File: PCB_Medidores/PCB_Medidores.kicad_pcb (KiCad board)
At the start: 2 copper layers, 85 x 56 mm, 20 parts, among them SW1 SW_Push, U1 SENO, U2 tp4056, U3 DS18B20, U4 ATmega8L-8PU, U5 EL814, U6 NRF24L01_Breakout, Y1 16MHz

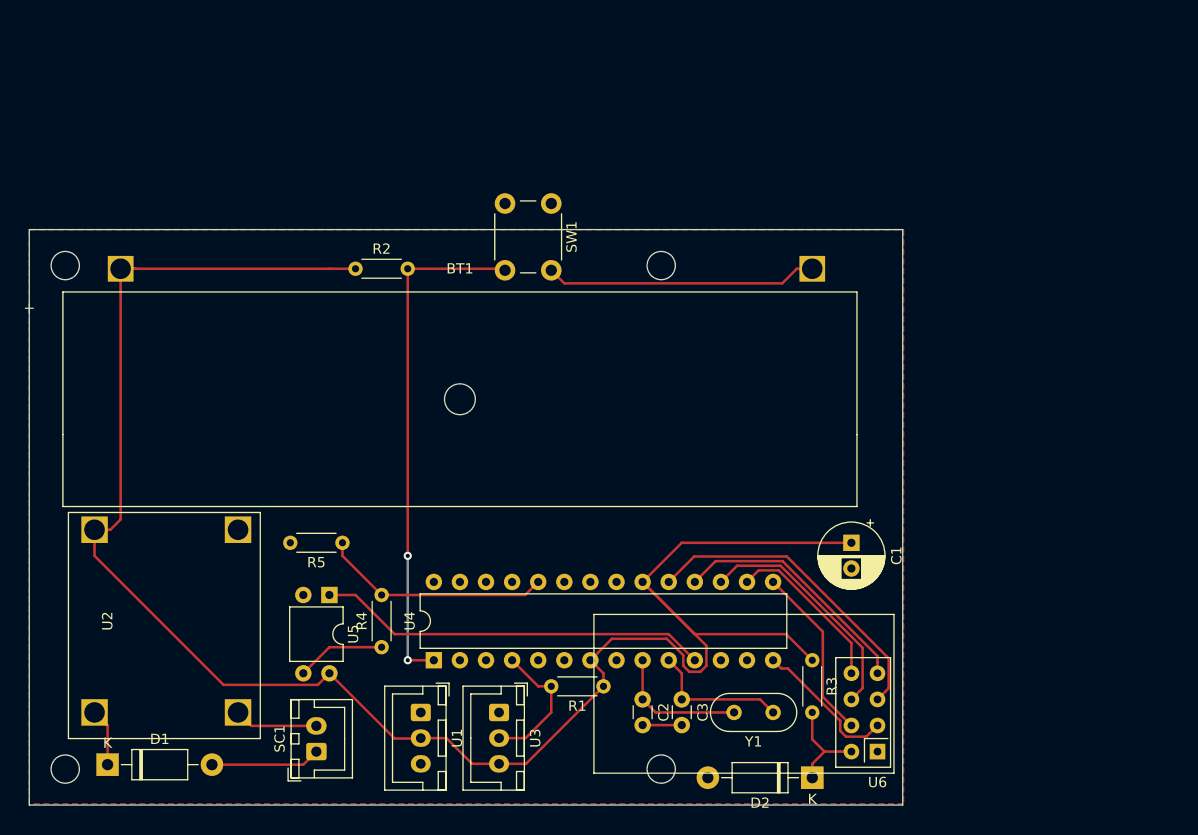
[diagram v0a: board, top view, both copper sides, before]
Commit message: [PCB Medidores e Correção]
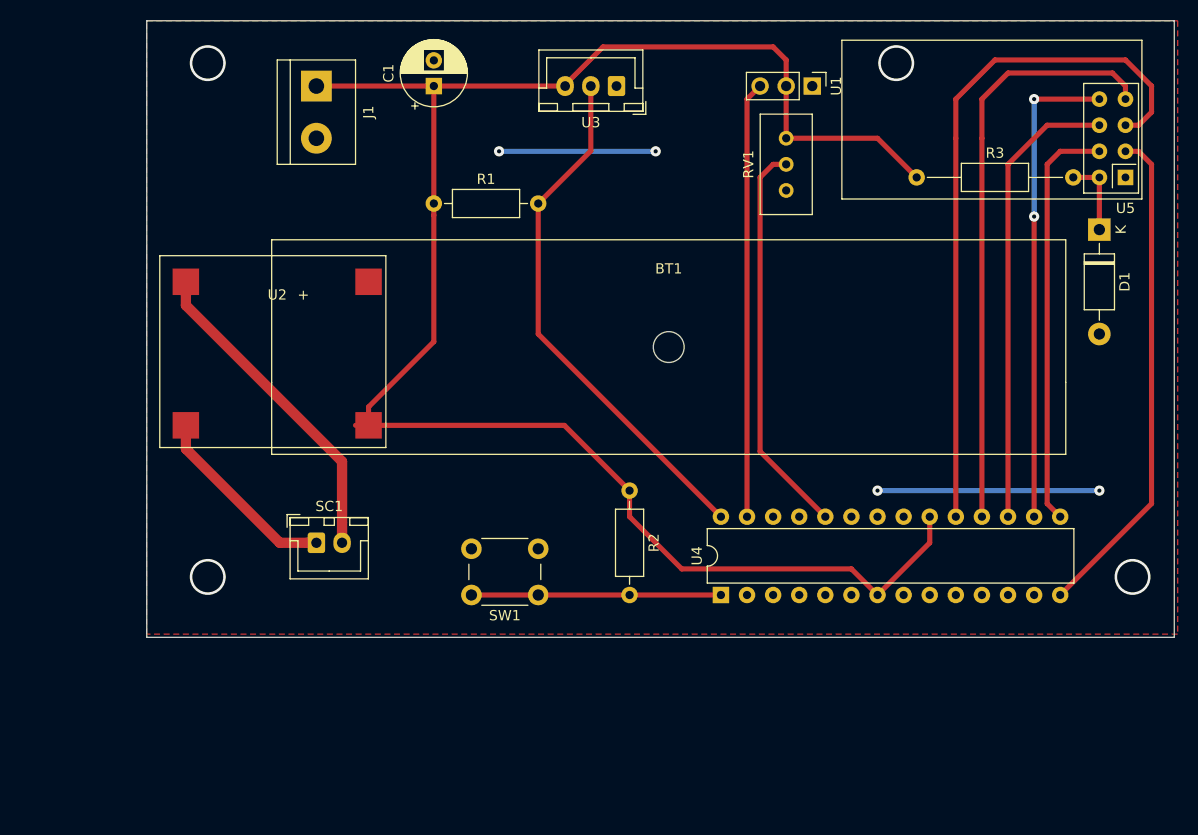
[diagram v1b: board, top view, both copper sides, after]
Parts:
- removed C2, C3: 22pF, Capacitor_THT:C_Disc_D3.0mm_W1.6mm_P2.50mm
- removed D2: 1N4728, Diode_THT:D_DO-41_SOD81_P10.16mm_Horizontal
- removed R4: 10k, Resistor_THT:R_Axial_DIN0204_L3.6mm_D1.6mm_P5.08mm_Horizontal
- removed R5: 33k, Resistor_THT:R_Axial_DIN0204_L3.6mm_D1.6mm_P5.08mm_Horizontal
- removed U6: NRF24L01_Breakout, RF_Module:nRF24L01_Breakout
- removed Y1: 16MHz, Crystal:Crystal_HC52-6mm_Vertical
- added J1: Screw_Terminal_01x02, TerminalBlock:TerminalBlock_bornier-2_P5.08mm, F.Cu at (115.6, 62.2)
- added RV1: R_POT_TRIM, Potentiometer_THT:Potentiometer_Bourns_3296W_Vertical, F.Cu at (161.3, 67.3)
- D1: value 1N4007 -> 1N4728
- R1, R2: footprint Resistor_THT:R_Axial_DIN0204_L3.6mm_D1.6mm_P5.08mm_Horizontal -> Resistor_THT:R_Axial_DIN0207_L6.3mm_D2.5mm_P10.16mm_Horizontal
- R3: footprint Resistor_THT:R_Axial_DIN0204_L3.6mm_D1.6mm_P5.08mm_Horizontal -> Resistor_THT:R_Axial_DIN0207_L6.3mm_D2.5mm_P15.24mm_Horizontal
- SW1: footprint Button_Switch_THT:SW_PUSH_6mm_H5mm -> Button_Switch_THT:SW_PUSH_6mm_H4.3mm
- U1: footprint Connector_JST:JST_XH_B3B-XH-A_1x03_P2.50mm_Vertical -> Connector_PinHeader_2.54mm:PinHeader_1x03_P2.54mm_Vertical
- U4: value ATmega8L-8PU -> ATmega328P-PU
- U5: value EL814 -> NRF24L01_Breakout; footprint Package_DIP:DIP-4_W7.62mm -> RF_Module:nRF24L01_Breakout
- moved D1 109.7 mm to (191.8, 76.2), turned to 270 degrees
- moved U5 87.5 mm to (194.3, 71.1), turned to 180 degrees
- moved U1 71.9 mm to (163.8, 62.2)
- moved U3 62.0 mm to (144.8, 62.2), turned to 180 degrees
- moved C1 60.2 mm to (127.0, 62.2), turned to 90 degrees
- moved R1 49.8 mm to (127.0, 73.7), turned to 0 degrees
- moved R3 48.1 mm to (174.0, 71.1), turned to 0 degrees
- moved U2 41.5 mm to (110.5, 78.7), turned to 0 degrees
- moved SW1 38.1 mm to (137.2, 111.8), turned to 180 degrees
- moved R2 34.3 mm to (146.1, 101.6), turned to 270 degrees
- moved U4 28.7 mm to (154.9, 111.8)
- moved BT1 20.9 mm to (149.9, 82.5)
- moved SC1 20.3 mm to (115.6, 106.7), turned to 0 degrees
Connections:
- D1 pad 2: Net-(D1-Pad2) -> GND
- R3 pad 2: Net-(D2-Pad1) -> Net-(D1-Pad1)
- SC1 pad 1: Net-(D1-Pad2) -> Net-(SC1-Pad1)
- SW1 pad 1: GND -> Net-(R2-Pad2)
- SW1 pad 2: Net-(R2-Pad2) -> GND
- U1 pad 3: Net-(U1-Pad3) -> A0
- U2 pad 1: Net-(D1-Pad1) -> Net-(SC1-Pad1)
- U4 pad 11: AT05 -> Net-(U4-Pad11)
- U4 pad 12: AT06 -> Net-(U4-Pad12)
- U4 pad 23: A0 -> Net-(U4-Pad23)
- U4 pad 27: Net-(U4-Pad27) -> A0
- U4 pad 28: Net-(U4-Pad28) -> AT02
- U4 pad 4: AT02 -> AT05
- U4 pad 5: Net-(U4-Pad5) -> AT06
- U5 pad 1: AT05 -> GND
- U5 pad 2: GND -> Net-(D1-Pad1)
- U5 pad 3: Net-(R4-Pad1) -> AT08
- U5 pad 4: +3V8 -> AT09
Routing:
- net A0: track 0.00 -> 42.4 mm
- net AT05: track 38.2 -> 0.00 mm
- net AT02: track 13.7 -> 51.4 mm
- net AT13: track 31.0 -> 67.9 mm
- net AT08: track 14.3 -> 48.7 mm
- net AT12: track 24.1 -> 57.5 mm
- net AT10: track 16.5 -> 47.0 mm, vias 0 -> 2
- net Net-(R2-Pad2): track 50.2 -> 24.3 mm, vias 2 -> 0
- net Net-(SC1-Pad2): track 8.16 -> 31.9 mm
- net AT09: track 17.1 -> 40.4 mm
- net AT11: track 23.2 -> 44.8 mm
- net Net-(SC1-Pad1): track 0.00 -> 18.8 mm
- net A1: track 22.4 -> 38.7 mm
- net Net-(U4-Pad10): track 13.8 -> 0.00 mm
- net Net-(U4-Pad9): track 13.2 -> 0.00 mm
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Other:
- board size 85 x 56 mm -> 100 x 60 mm
